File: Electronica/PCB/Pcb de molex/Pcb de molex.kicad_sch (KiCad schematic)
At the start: 11 parts, among them J1 Conn_01x05, J2 Conn_01x05, J3 Conn_01x05, U1 ULTRASONICO1, U2 ULTRASONICO2, U3 ULTRASONICO3, U4 ULTRASONICO4, U5 ULTRASONICO5

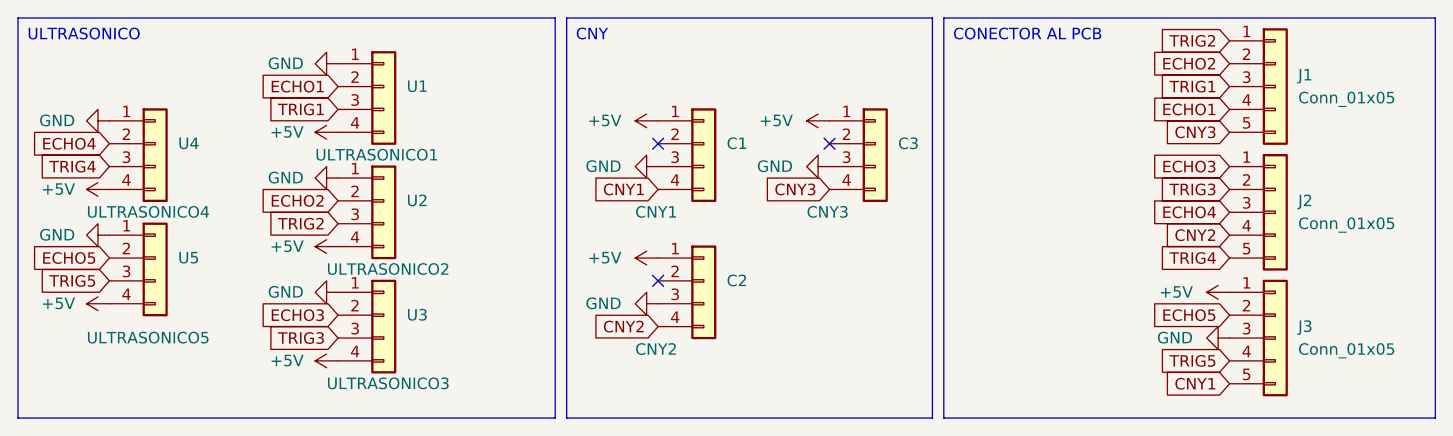
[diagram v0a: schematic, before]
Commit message: ?
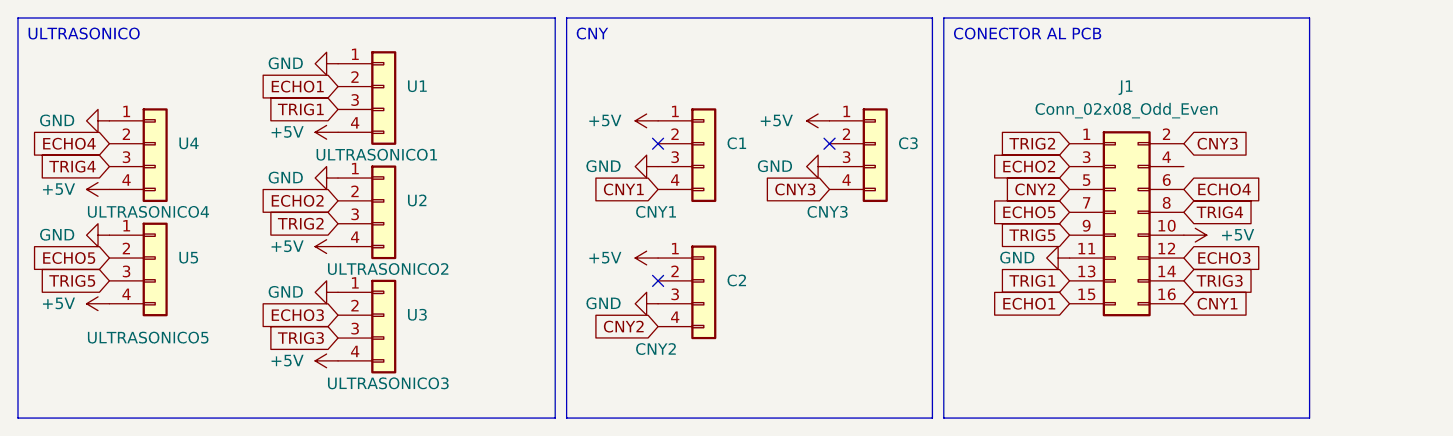
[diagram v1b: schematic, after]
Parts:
- removed J1, J2, J3: Conn_01x05, Connector_PinSocket_2.54mm:PinSocket_1x05_P2.54mm_Vertical, symbol Connector_Generic:Conn_01x05
- added J1: Conn_02x08_Odd_Even, Connector_PinHeader_2.54mm:PinHeader_2x08_P2.54mm_Horizontal, symbol Connector_Generic:Conn_02x08_Odd_Even
- U5: footprint Connector_PinHeader_2.54mm:PinHeader_1x04_P2.54mm_Horizontal -> Connector_PinHeader_2.54mm:PinHeader_1x04_P2.54mm_Vertical
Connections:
- net +5V: now also J1.10 (Pin_10)
- net CNY1: now also J1.16 (Pin_16)
- net CNY2: now also J1.5 (Pin_5)
- net CNY3: now also J1.2 (Pin_2)
- net ECHO1: now also J1.15 (Pin_15)
- net ECHO2: now also J1.3 (Pin_3)
- net ECHO3: now also J1.12 (Pin_12)
- net ECHO4: now also J1.6 (Pin_6)
- net ECHO5: now also J1.7 (Pin_7)
- net GND: now also J1.11 (Pin_11)
- net TRIG1: now also J1.13 (Pin_13)
- net TRIG2: now also J1.1 (Pin_1)
- net TRIG3: now also J1.14 (Pin_14)
- net TRIG4: now also J1.8 (Pin_8)
- net TRIG5: now also J1.9 (Pin_9)
